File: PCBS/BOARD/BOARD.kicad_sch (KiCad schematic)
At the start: 79 parts, among them J38 USB_B_Micro, Q1 NMOS, U1 ATmega88PB-A, U2 SN74HC574DWR

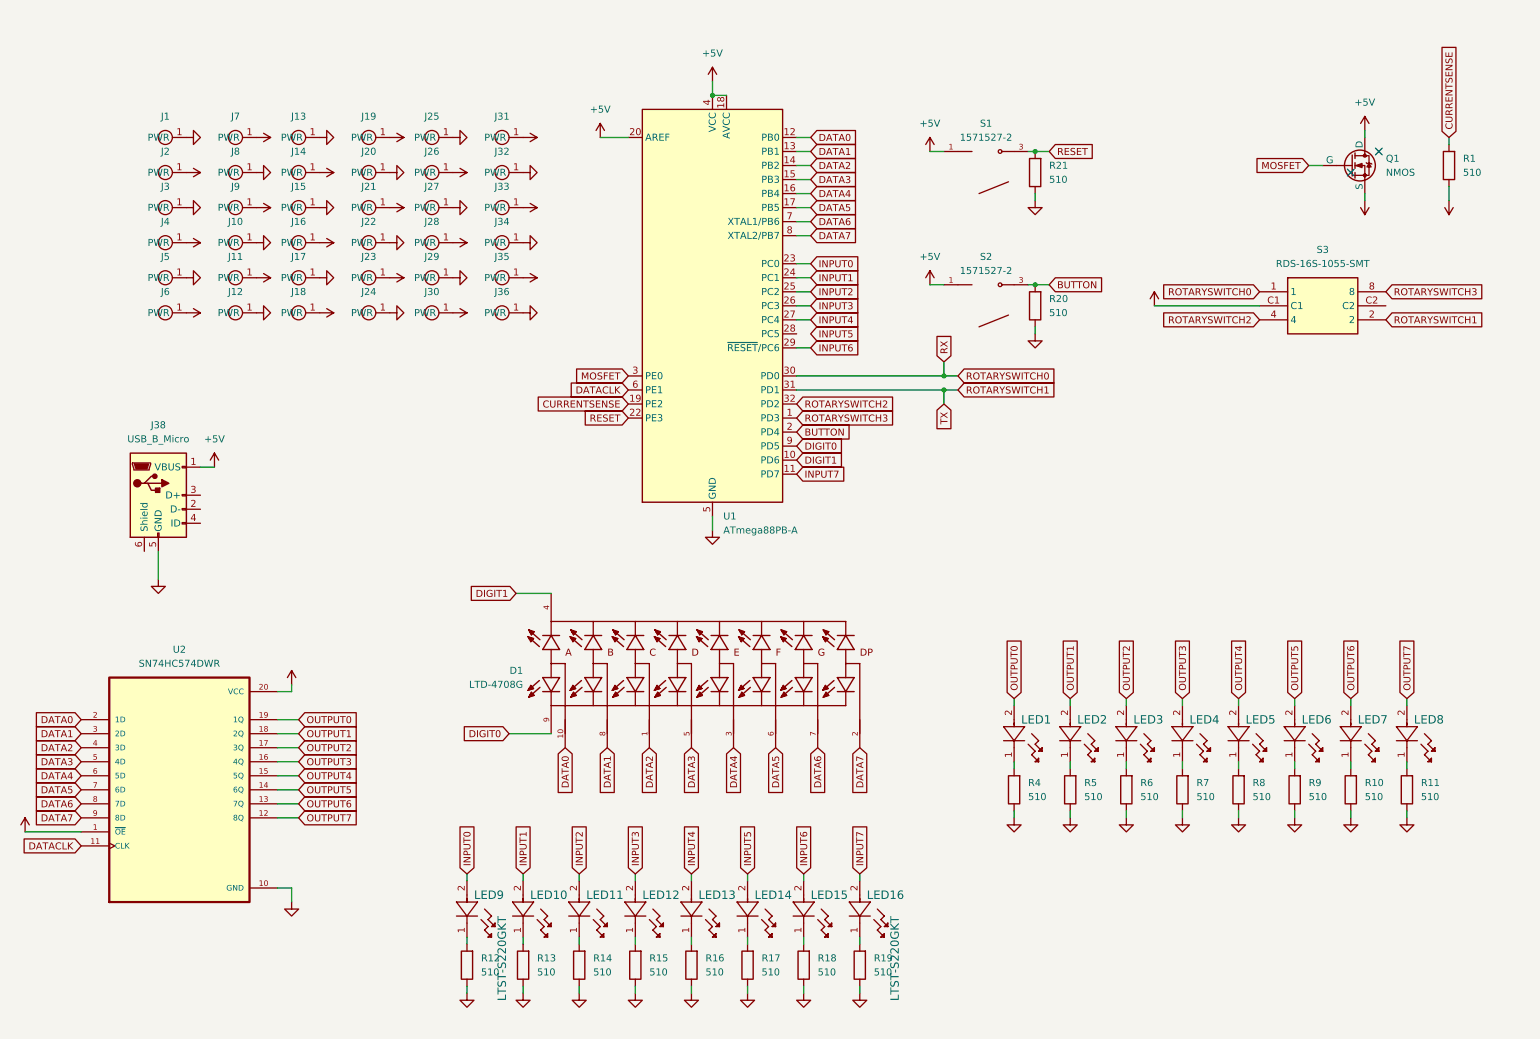
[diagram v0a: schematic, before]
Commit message: Rev1 board/mux/switches/output
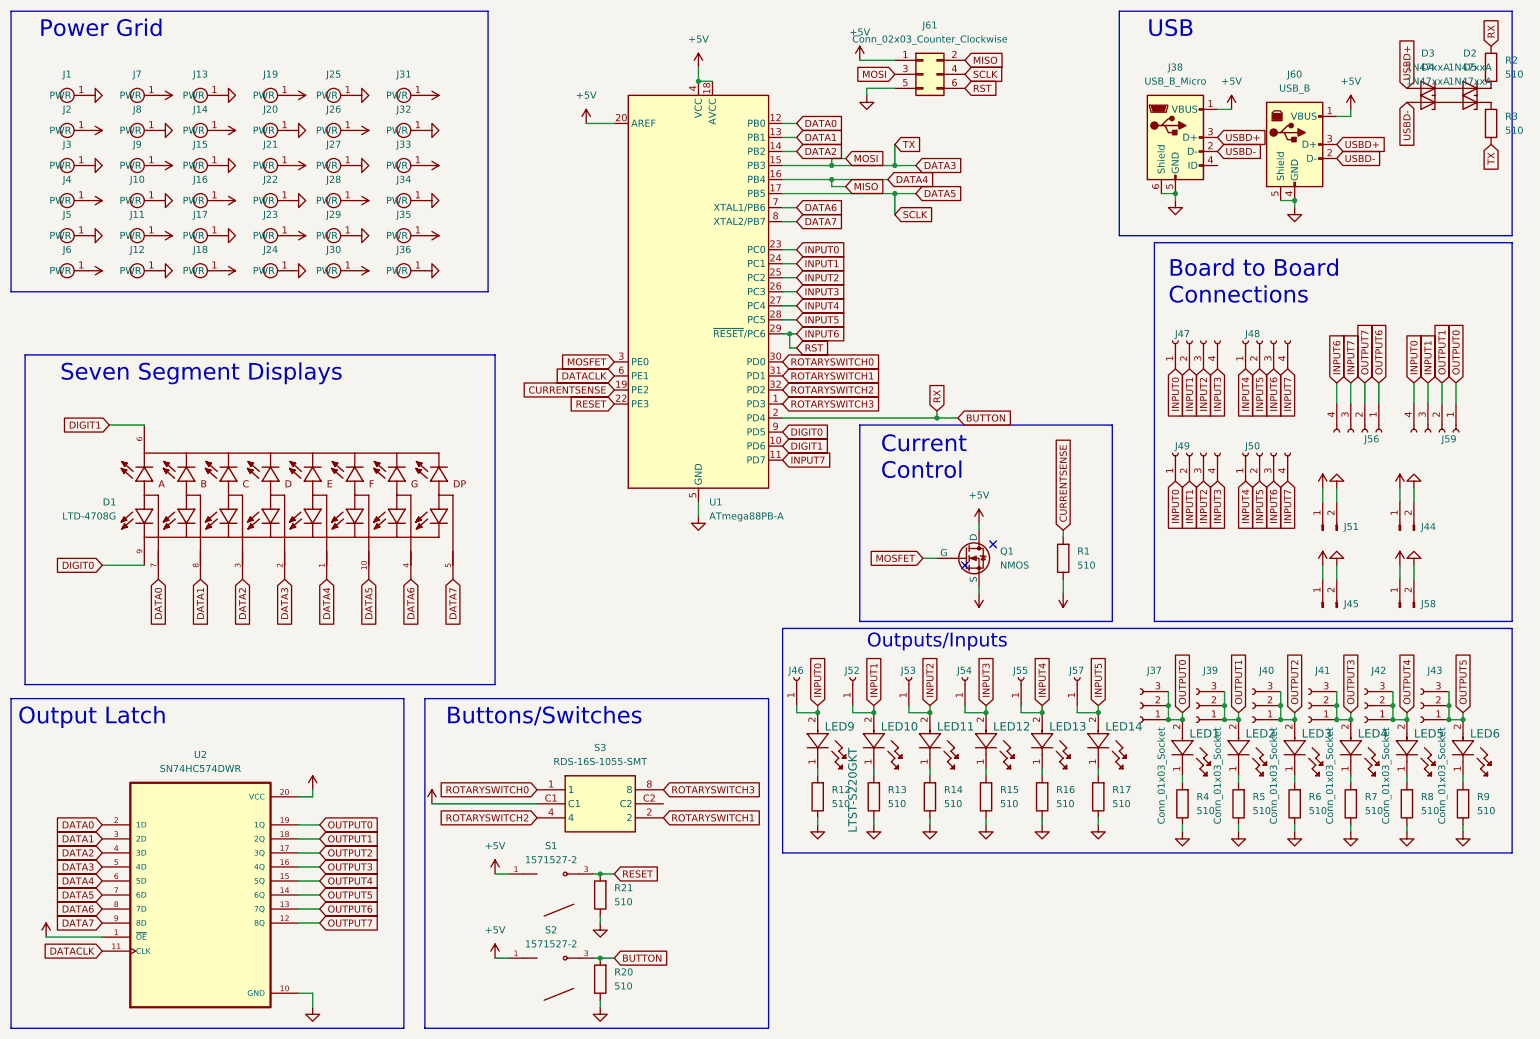
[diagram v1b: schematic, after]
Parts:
- removed LED15, LED16, LED7, LED8: LTST-S220GKT, LED_LTST-S220GKT_LTO, symbol DigitalLogicLibrary:LTST-S220GKT
- removed R10, R11, R18, R19: 510, Resistor_SMD:R_0805_2012Metric_Pad1.20x1.40mm_HandSolder, symbol Device:R
- added D2, D3, D4, D5: 1N47xxA, Diode_THT:D_DO-41_SOD81_P10.16mm_Horizontal, symbol Diode:1N47xxA
- added J37, J39, J40, J41, J42, J43: Conn_01x03_Socket, DigitalLogicFootprints:PinHeader_1x03_P2.54mm_Vertical, symbol DigitalLogicLibrary:Conn_01x03_Socket
- added J44, J45, J51, J58: Conn_01x02_Pin, DigitalLogicFootprints:PinHeader_1x02_P2.54mm_Horizontal, symbol Connector:Conn_01x02_Pin
- added J46, J52, J53, J54, J55, J57: Conn_01x01_Socket, Connector_PinSocket_2.54mm:PinSocket_1x01_P2.54mm_Vertical, symbol DigitalLogicLibrary:Conn_01x01_Socket
- added J47, J48, J49, J50, J56, J59: Conn_01x04_Socket, DigitalLogicFootprints:PinHeader_1x04_P2.54mm_Horizontal, symbol Connector:Conn_01x04_Socket
- added J60: USB_B, Connector_USB:USB_B_OST_USB-B1HSxx_Horizontal, symbol Connector:USB_B
- added J61: Conn_02x03_Counter_Clockwise, Connector_PinSocket_2.54mm:PinSocket_2x03_P2.54mm_Vertical, symbol Connector_Generic:Conn_02x03_Odd_Even
- added R2, R3: 510, Resistor_SMD:R_0805_2012Metric_Pad1.20x1.40mm_HandSolder, symbol Device:R
- J38: footprint Connector_USB:USB_Micro-AB_Molex_47590-0001 -> Connector_USB:USB_Micro-B_Amphenol_10118194_Horizontal
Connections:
- net +5V: now also J60.1 (VBUS), J61.1 (Pin_1)
- net BUTTON: now also R2.1
- net DATA0: now also D1.7; no longer D1.10
- net DATA2: now also D1.3; no longer D1.1
- net DATA3: now also D1.2, J61.3 (Pin_3), R3.2; no longer D1.5
- net DATA4: now also D1.1, J61.2 (Pin_2); no longer D1.3
- net DATA5: now also D1.10, J61.4 (Pin_4); no longer D1.6
- net DATA6: now also D1.4; no longer D1.7
- net DATA7: now also D1.5; no longer D1.2
- net DIGIT1: now also D1.6; no longer D1.4
- net GND: now also J38.6 (Shield), J44.2 (Pin_2), J45.2 (Pin_2), J51.2 (Pin_2), J58.2 (Pin_2), J60.4 (GND), J60.5 (Shield), J61.5 (Pin_5)
- net INPUT0: now also J46.1 (Pin_1), J47.1 (Pin_1), J49.1 (Pin_1), J59.4 (Pin_4)
- net INPUT1: now also J47.2 (Pin_2), J49.2 (Pin_2), J52.1 (Pin_1), J59.3 (Pin_3)
- net INPUT2: now also J47.3 (Pin_3), J49.3 (Pin_3), J53.1 (Pin_1)
- net INPUT3: now also J47.4 (Pin_4), J49.4 (Pin_4), J54.1 (Pin_1)
- net INPUT4: now also J48.1 (Pin_1), J50.1 (Pin_1), J55.1 (Pin_1)
- net INPUT5: now also U1.28 (PC5), J48.2 (Pin_2), J50.2 (Pin_2), J57.1 (Pin_1)
- net INPUT6: now also J48.3 (Pin_3), J50.3 (Pin_3), J56.4 (Pin_4), J61.6 (Pin_6)
- net INPUT7: now also J48.4 (Pin_4), J50.4 (Pin_4), J56.3 (Pin_3)
- net OUTPUT0: now also J37.1 (Pin_1), J37.2 (Pin_2), J37.3 (Pin_3), J59.1 (Pin_1)
- net OUTPUT1: now also J39.1 (Pin_1), J39.2 (Pin_2), J39.3 (Pin_3), J59.2 (Pin_2)
- net OUTPUT2: now also J40.1 (Pin_1), J40.2 (Pin_2), J40.3 (Pin_3)
- net OUTPUT3: now also J41.1 (Pin_1), J41.2 (Pin_2), J41.3 (Pin_3)
- net OUTPUT4: now also J42.1 (Pin_1), J42.2 (Pin_2), J42.3 (Pin_3)
- net OUTPUT5: now also J43.1 (Pin_1), J43.2 (Pin_2), J43.3 (Pin_3)
- net OUTPUT6: now also J56.1 (Pin_1)
- net OUTPUT7: now also J56.2 (Pin_2)
- net VCC: now also J44.1 (Pin_1), J45.1 (Pin_1), J51.1 (Pin_1), J58.1 (Pin_1)
- net USBD-: now reaches J38.2 (D-)
- net USBD-: now also D4.2 (A), J60.2 (D-)
- net USBD+: now reaches J38.3 (D+)
- net USBD+: now also D3.2 (A), J60.3 (D+)
- new net: D2.2 (A), D3.1 (K)
- new net: D2.1 (K), R2.2
- new net: D5.1 (K), R3.1
- new net: D4.1 (K), D5.2 (A)
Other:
- note added: "Board to Board Connections"
- note added: "Buttons/Switches"
- note added: "Current Control"
- note added: "Output Latch"
- note added: "Outputs/Inputs"
- note added: "Power Grid"
- note added: "Seven Segment Displays"
- note added: "USB"
- moved on the sheet: D1, J1, J10, J11, J12, J13, J14, J15, J16, J17, J18, J19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
